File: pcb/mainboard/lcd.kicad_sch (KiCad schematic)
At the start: 15 parts

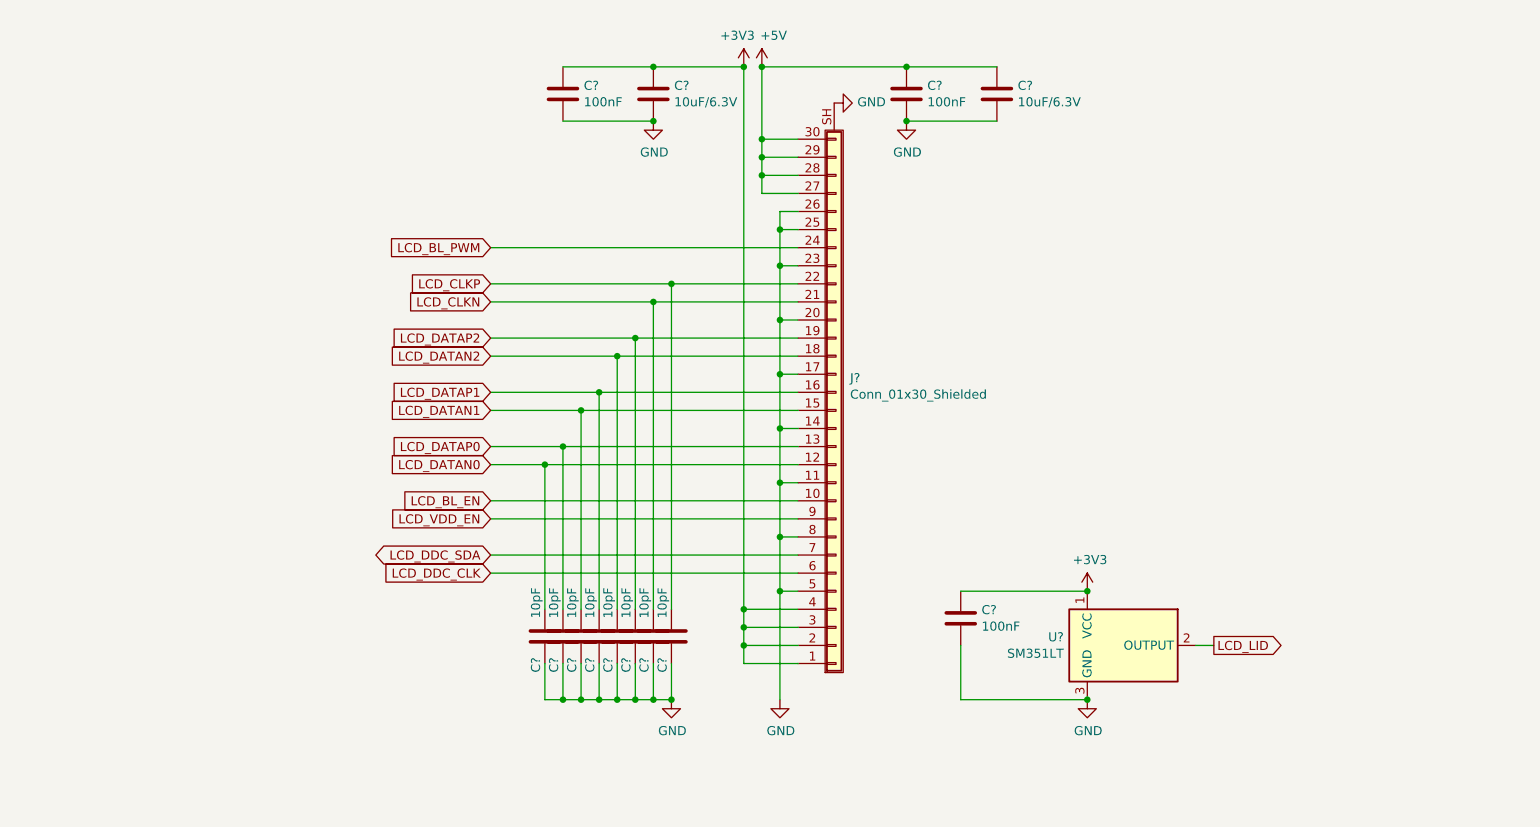
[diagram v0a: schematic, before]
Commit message: - Upgrade KiCad to latest version - Working on PM circuits - Initial USB Type-C support - Initial support for LCD
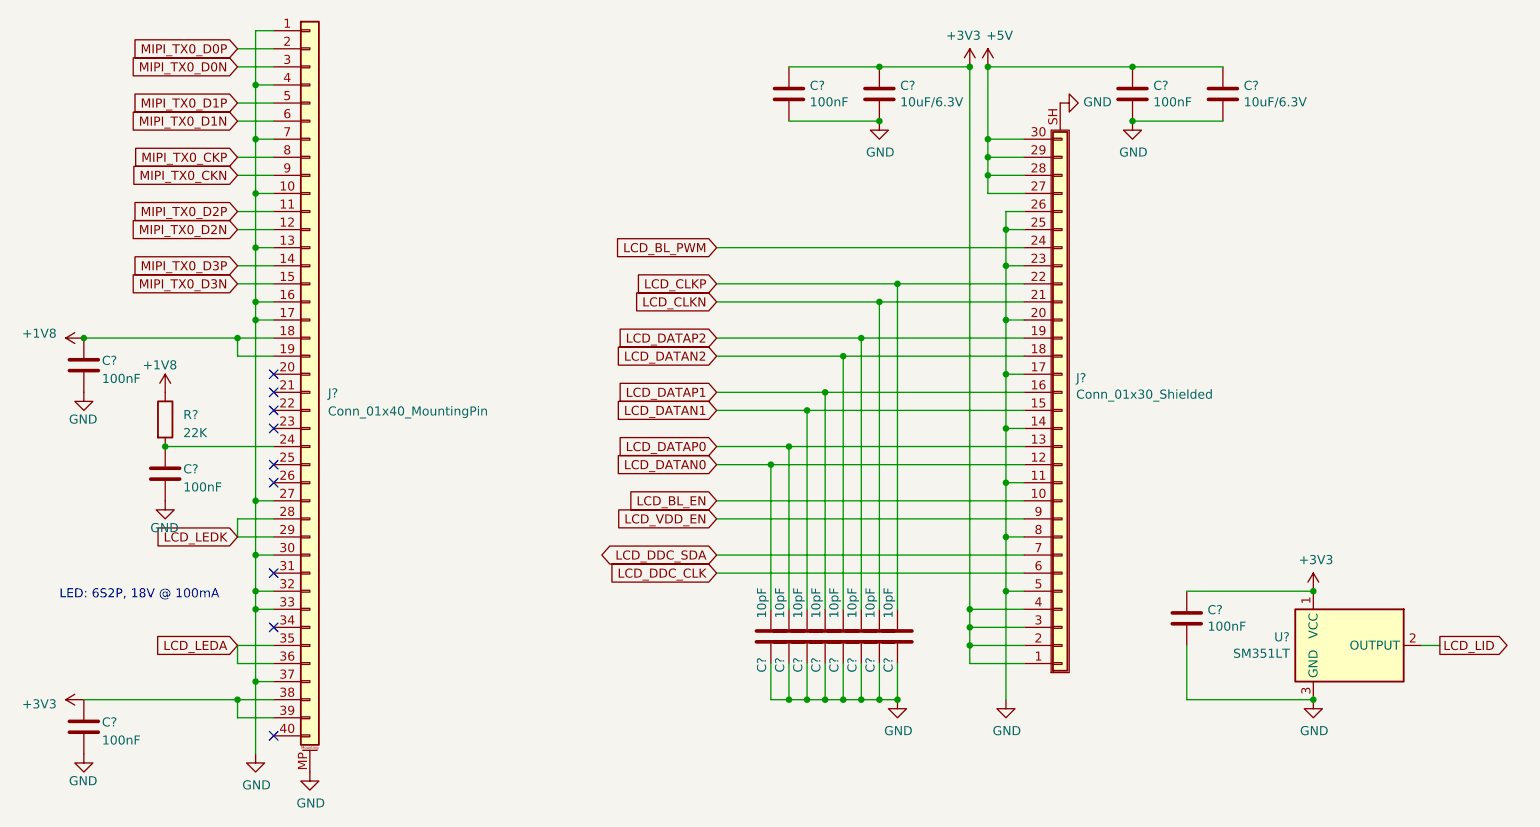
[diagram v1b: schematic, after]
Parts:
- added C? (x3): 100nF, symbol Device:C
- added J?: Conn_01x40_MountingPin, symbol Connector_Generic_MountingPin:Conn_01x40_MountingPin
- added R?: 22K, Resistor_SMD:R_0402_1005Metric, symbol Device:R
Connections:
- net +3V3: now also C?.1, J?.38 (Pin_38), J?.39 (Pin_39)
- net GND: now also C?.2, C?.2, C?.2, J?.1 (Pin_1), J?.10 (Pin_10), J?.13 (Pin_13), J?.16 (Pin_16), J?.17 (Pin_17), J?.27 (Pin_27), J?.30 (Pin_30), J?.32 (Pin_32), J?.33 (Pin_33), J?.37 (Pin_37), J?.4 (Pin_4), J?.7 (Pin_7), J?.MP (MountPin)
- new net: C?.1, J?.24 (Pin_24), R?.2
- new net +1V8: C?.1, J?.18 (Pin_18), J?.19 (Pin_19), R?.1
- new net LCD_LEDA: J?.35 (Pin_35), J?.36 (Pin_36)
- new net LCD_LEDK: J?.28 (Pin_28), J?.29 (Pin_29)
- new net MIPI_TX0_CKN: J?.9 (Pin_9)
- new net MIPI_TX0_CKP: J?.8 (Pin_8)
- new net MIPI_TX0_D0N: J?.3 (Pin_3)
- new net MIPI_TX0_D0P: J?.2 (Pin_2)
- new net MIPI_TX0_D1N: J?.6 (Pin_6)
- new net MIPI_TX0_D1P: J?.5 (Pin_5)
- new net MIPI_TX0_D2N: J?.12 (Pin_12)
- new net MIPI_TX0_D2P: J?.11 (Pin_11)
- new net MIPI_TX0_D3N: J?.15 (Pin_15)
- new net MIPI_TX0_D3P: J?.14 (Pin_14)
- no-connect marks 0 -> 9
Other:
- note added: "LED: 6S2P, 18V @ 100mA"
- moved on the sheet: C?, J?, U?

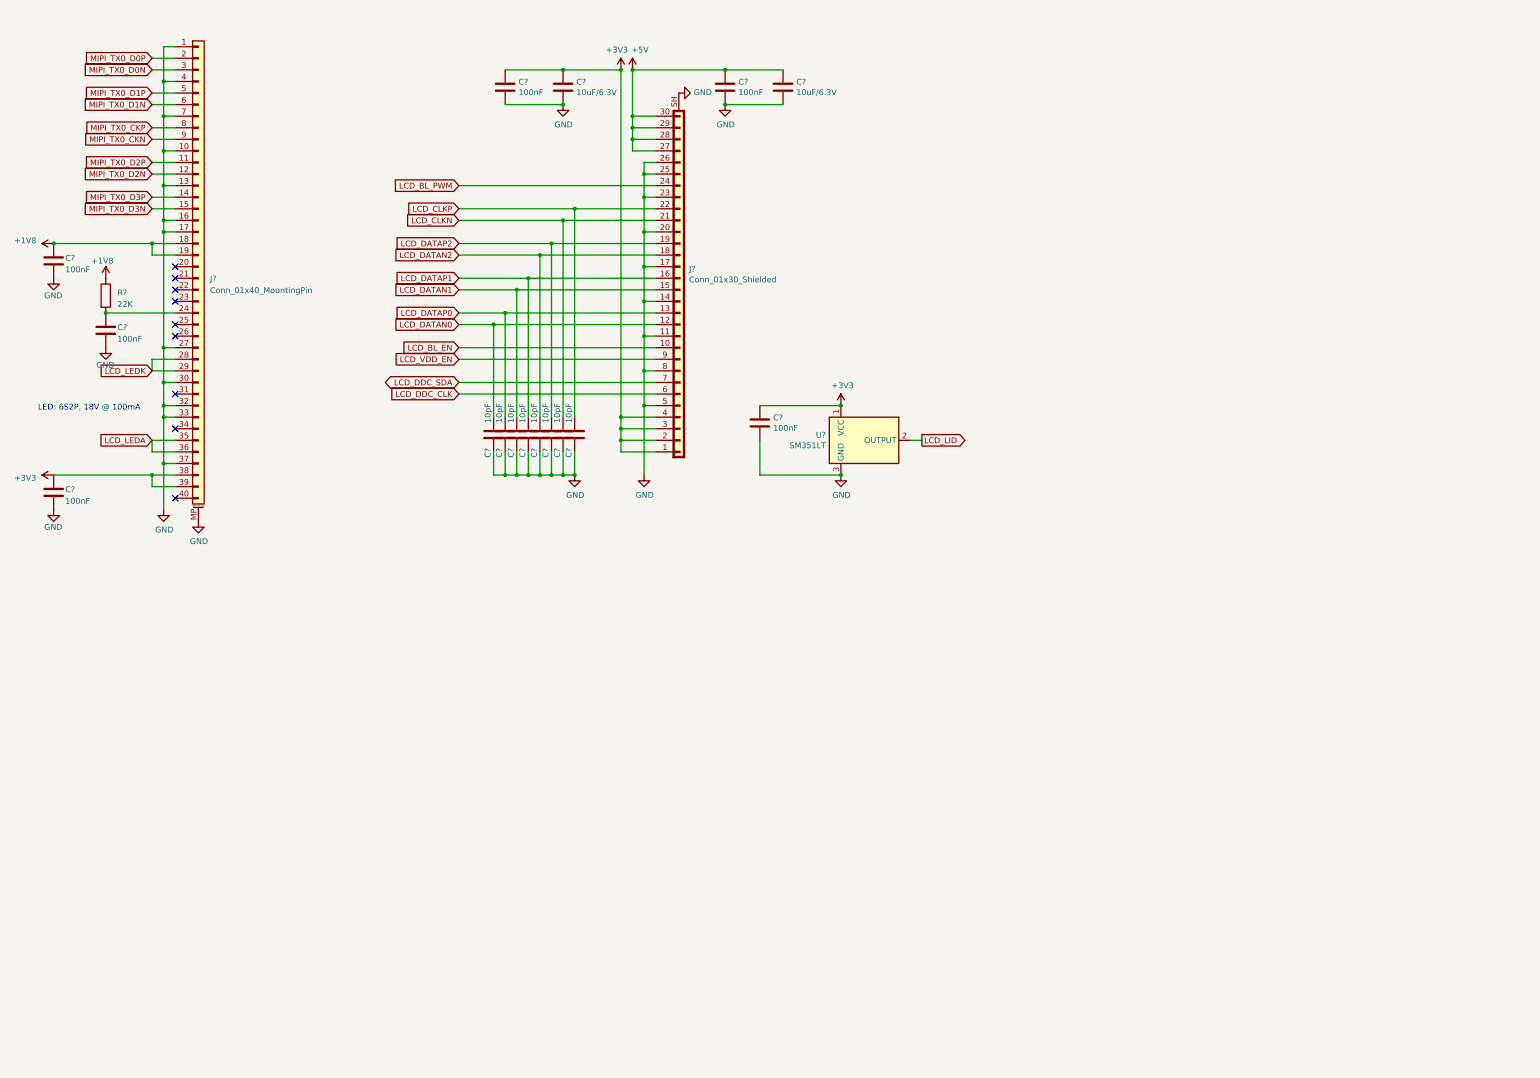
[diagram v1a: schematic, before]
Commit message: - pcb: working on r0p1 sch
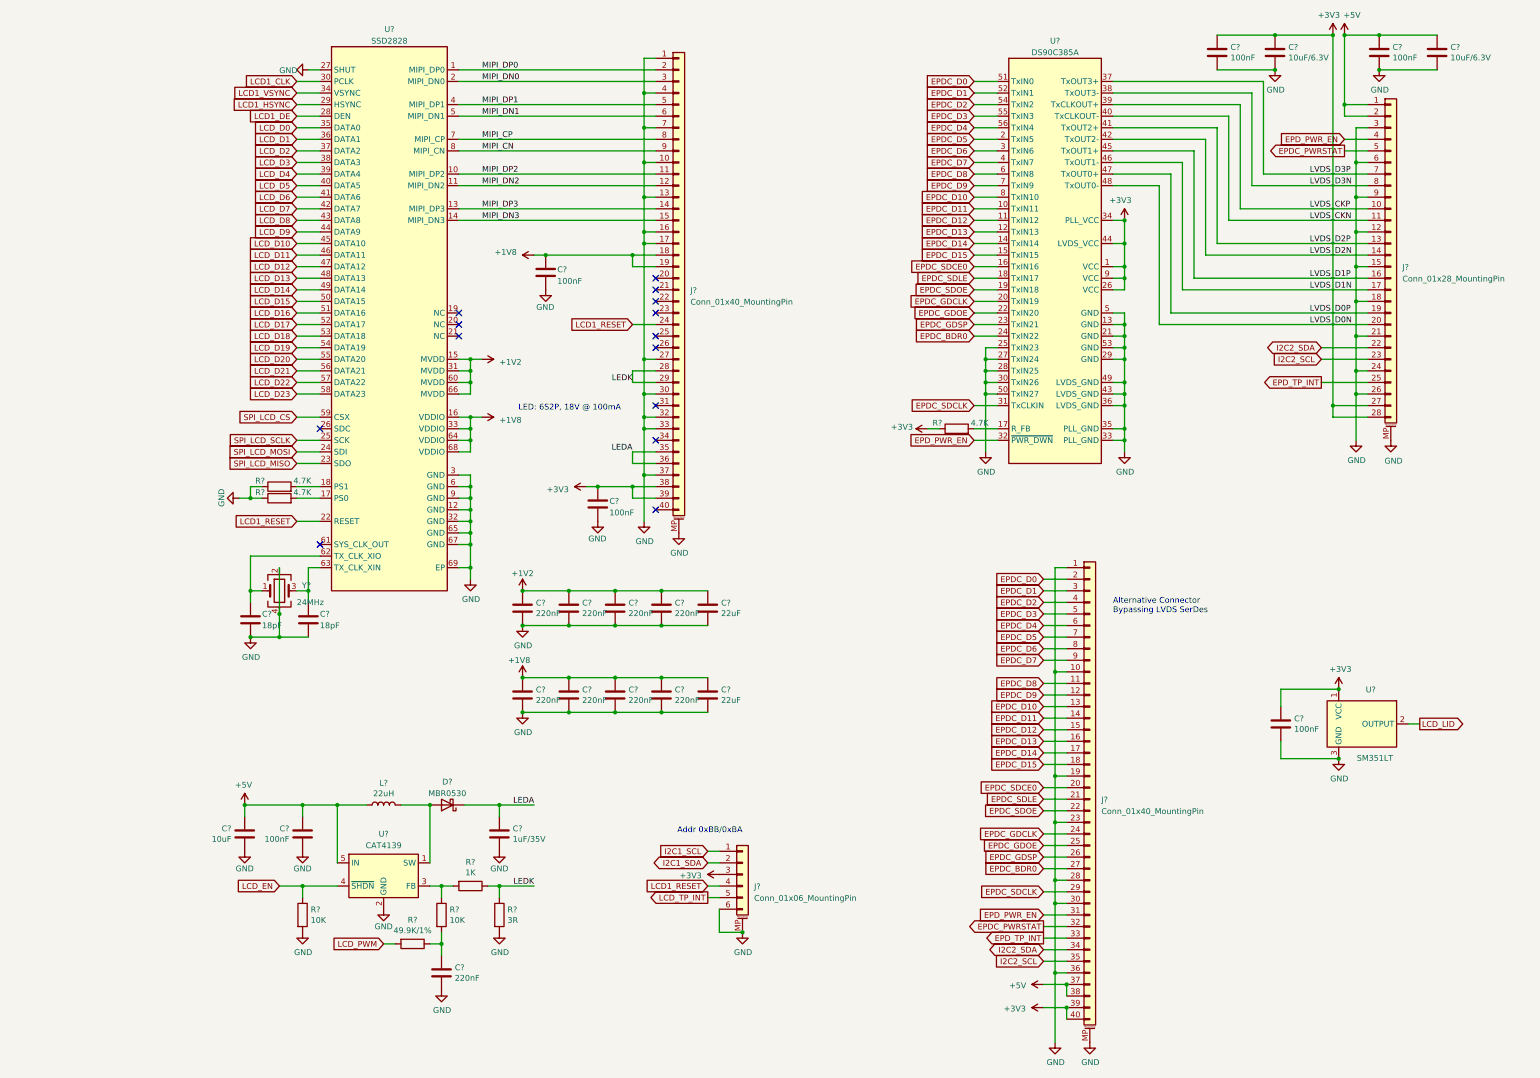
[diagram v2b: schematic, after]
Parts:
- removed C? (x8): 10pF, symbol Device:C
- removed C?: 100nF, symbol Device:C
- removed J?: Conn_01x30_Shielded, symbol Connector_Generic_Shielded:Conn_01x30_Shielded
- removed R?: 22K, Resistor_SMD:R_0402_1005Metric, symbol Device:R
- added C? (x9): 220nF, Capacitor_SMD:C_0402_1005Metric, symbol Device:C
- added C? (x2): 22uF, Capacitor_SMD:C_0603_1608Metric, symbol Device:C
- added C? (x2): 18pF, Capacitor_SMD:C_0603_1608Metric, symbol Device:C
- added C?: 1uF/35V, Capacitor_SMD:C_0603_1608Metric, symbol Device:C
- added C?: 100nF, Capacitor_SMD:C_0402_1005Metric, symbol Device:C
- added C?: 10uF, Capacitor_SMD:C_0603_1608Metric, symbol Device:C
- added D?: MBR0530, Diode_SMD:D_SOD-123, symbol Diode:MBR0530
- added J?: Conn_01x06_MountingPin, symbol Connector_Generic_MountingPin:Conn_01x06_MountingPin
- added J?: Conn_01x28_MountingPin, symbol Connector_Generic_MountingPin:Conn_01x28_MountingPin
- added J?: Conn_01x40_MountingPin, symbol Connector_Generic_MountingPin:Conn_01x40_MountingPin
- added L?: 22uH, Inductor_SMD:L_Vishay_IHLP-1212, symbol Device:L
- added R? (x3): 4.7K, Resistor_SMD:R_0402_1005Metric, symbol Device:R
- added R? (x2): 10K, Resistor_SMD:R_0402_1005Metric, symbol Device:R
- added R?: 3R, Resistor_SMD:R_0402_1005Metric, symbol Device:R
- added R?: 1K, Resistor_SMD:R_0402_1005Metric, symbol Device:R
- added R?: 49.9K/1%, Resistor_SMD:R_0402_1005Metric, symbol Device:R
- added U?: DS90C385A, Package_SO:TSSOP-56_6.1x14mm_P0.5mm, symbol symbols:DS90C385A
- added U?: CAT4139, Package_TO_SOT_SMD:SOT-23-5, symbol Regulator_Switching:AP3012
- added U?: SSD2828, Package_DFN_QFN:QFN-68-1EP_8x8mm_P0.4mm_EP5.2x5.2mm_ThermalVias, symbol symbols:SSD2828
- added Y?: 24MHz, Crystal:Crystal_SMD_3225-4Pin_3.2x2.5mm, symbol Device:Crystal_GND24
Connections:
- net +1V8: now also C?.1, C?.1, C?.1, C?.1, C?.1, U?.16 (VDDIO), U?.33 (VDDIO), U?.64 (VDDIO), U?.68 (VDDIO)
- net +3V3: now also J?.27 (Pin_27), J?.28 (Pin_28), J?.3 (Pin_3), J?.39 (Pin_39), J?.40 (Pin_40), R?.1, U?.1 (VCC), U?.26 (VCC), U?.34 (PLL_VCC), U?.44 (LVDS_VCC), U?.9 (VCC)
- net +5V: now also C?.2, C?.2, J?.1 (Pin_1), J?.2 (Pin_2), J?.37 (Pin_37), J?.38 (Pin_38), L?.1, U?.5 (IN)
- net GND: now also C?.1, C?.1, C?.1, C?.1, C?.1, C?.1, C?.2, C?.2, C?.2, C?.2, C?.2, C?.2, C?.2, C?.2, C?.2, C?.2, J?.1 (Pin_1), J?.10 (Pin_10), J?.12 (Pin_12), J?.15 (Pin_15), J?.18 (Pin_18), J?.19 (Pin_19), J?.21 (Pin_21), J?.23 (Pin_23), J?.24 (Pin_24), J?.26 (Pin_26), J?.28 (Pin_28), J?.3 (Pin_3), J?.30 (Pin_30), J?.36 (Pin_36), J?.6 (Pin_6), J?.6 (Pin_6), J?.9 (Pin_9), J?.MP (MountPin), J?.MP (MountPin), J?.MP (MountPin), R?.1, R?.1, R?.2, R?.2, U?.12 (GND), U?.13 (GND), U?.2 (GND), U?.21 (GND), U?.25 (TxIN23), U?.27 (SHUT), U?.27 (TxIN24), U?.28 (TxIN25), U?.29 (GND), U?.3 (GND), U?.30 (TxIN26), U?.32 (GND), U?.33 (PLL_GND), U?.35 (PLL_GND), U?.36 (LVDS_GND), U?.43 (LVDS_GND), U?.49 (LVDS_GND), U?.5 (GND), U?.50 (TxIN27), U?.53 (GND), U?.6 (GND), U?.65 (GND), U?.67 (GND), U?.69 (EP), U?.9 (GND), Y?.2, Y?.4
- net LCD1_RESET: now reaches J?.24 (Pin_24)
- net LCD1_RESET: now also J?.4 (Pin_4), U?.22 (RESET)
- net LCD_LEDA renamed LEDA
- net LEDA: now also C?.2, D?.1 (K)
- net LCD_LEDK renamed LEDK
- net LEDK: now also R?.1, R?.1
- net MIPI_TX0_CKN renamed MIPI_CN
- net MIPI_CN: now also U?.8 (MIPI_CN)
- net MIPI_TX0_CKP renamed MIPI_CP
- net MIPI_CP: now also U?.7 (MIPI_CP)
- net MIPI_TX0_D0N renamed MIPI_DN0
- net MIPI_DN0: now also U?.2 (MIPI_DN0)
- net MIPI_TX0_D0P renamed MIPI_DP0
- net MIPI_DP0: now also U?.1 (MIPI_DP0)
- net MIPI_TX0_D1N renamed MIPI_DN1
- net MIPI_DN1: now also U?.5 (MIPI_DN1)
- net MIPI_TX0_D1P renamed MIPI_DP1
- net MIPI_DP1: now also U?.4 (MIPI_DP1)
- net MIPI_TX0_D2N renamed MIPI_DN2
- net MIPI_DN2: now also U?.11 (MIPI_DN2)
- net MIPI_TX0_D2P renamed MIPI_DP2
- net MIPI_DP2: now also U?.10 (MIPI_DP2)
- net MIPI_TX0_D3N renamed MIPI_DN3
- net MIPI_DN3: now also U?.14 (MIPI_DN3)
- net MIPI_TX0_D3P renamed MIPI_DP3
- net MIPI_DP3: now also U?.13 (MIPI_DP3)
- new net: R?.2, U?.18 (PS1)
- new net: R?.2, U?.17 (R_FB)
- new net: D?.2 (A), L?.2, U?.1 (SW)
- new net: R?.1, R?.2, U?.3 (FB)
- new net: C?.2, R?.1, R?.2
- new net: C?.2, U?.63 (TX_CLK_XIN), Y?.3
- new net: C?.2, U?.62 (TX_CLK_XIO), Y?.1
- new net: R?.2, U?.17 (PS0)
- new net +1V2: C?.1, C?.1, C?.1, C?.1, C?.1, U?.15 (MVDD), U?.31 (MVDD), U?.60 (MVDD), U?.66 (MVDD)
- new net EPDC_BDR0: J?.27 (Pin_27), U?.24 (TxIN22)
- new net EPDC_D0: J?.2 (Pin_2), U?.51 (TxIN0)
- new net EPDC_D1: J?.3 (Pin_3), U?.52 (TxIN1)
- new net EPDC_D10: J?.13 (Pin_13), U?.8 (TxIN10)
- new net EPDC_D11: J?.14 (Pin_14), U?.10 (TxIN11)
- new net EPDC_D12: J?.15 (Pin_15), U?.11 (TxIN12)
- new net EPDC_D13: J?.16 (Pin_16), U?.12 (TxIN13)
- new net EPDC_D14: J?.17 (Pin_17), U?.14 (TxIN14)
- new net EPDC_D15: J?.18 (Pin_18), U?.15 (TxIN15)
- new net EPDC_D2: J?.4 (Pin_4), U?.54 (TxIN2)
- new net EPDC_D3: J?.5 (Pin_5), U?.55 (TxIN3)
- new net EPDC_D4: J?.6 (Pin_6), U?.56 (TxIN4)
- new net EPDC_D5: J?.7 (Pin_7), U?.2 (TxIN5)
- new net EPDC_D6: J?.8 (Pin_8), U?.3 (TxIN6)
- new net EPDC_D7: J?.9 (Pin_9), U?.4 (TxIN7)
- new net EPDC_D8: J?.11 (Pin_11), U?.6 (TxIN8)
- new net EPDC_D9: J?.12 (Pin_12), U?.7 (TxIN9)
- new net EPDC_GDCLK: J?.24 (Pin_24), U?.20 (TxIN19)
- new net EPDC_GDOE: J?.25 (Pin_25), U?.22 (TxIN20)
- new net EPDC_GDSP: J?.26 (Pin_26), U?.23 (TxIN21)
- new net EPDC_PWRSTAT: J?.32 (Pin_32), J?.5 (Pin_5)
- new net EPDC_SDCE0: J?.20 (Pin_20), U?.16 (TxIN16)
- new net EPDC_SDCLK: J?.29 (Pin_29), U?.31 (TxCLKIN)
- new net EPDC_SDLE: J?.21 (Pin_21), U?.18 (TxIN17)
- new net EPDC_SDOE: J?.22 (Pin_22), U?.19 (TxIN18)
- new net EPD_PWR_EN: J?.31 (Pin_31), J?.4 (Pin_4), U?.32 (~PWR_DWN)
- new net EPD_TP_INT: J?.25 (Pin_25), J?.33 (Pin_33)
- new net I2C1_SCL: J?.1 (Pin_1)
- new net I2C1_SDA: J?.2 (Pin_2)
- new net I2C2_SCL: J?.23 (Pin_23), J?.35 (Pin_35)
- new net I2C2_SDA: J?.22 (Pin_22), J?.34 (Pin_34)
- new net LCD1_CLK: U?.30 (PCLK)
- new net LCD1_DE: U?.28 (DEN)
- new net LCD1_HSYNC: U?.29 (HSYNC)
- new net LCD1_VSYNC: U?.34 (VSYNC)
- new net LCD_D0: U?.35 (DATA0)
- new net LCD_D1: U?.36 (DATA1)
- new net LCD_D10: U?.45 (DATA10)
- new net LCD_D11: U?.46 (DATA11)
- new net LCD_D12: U?.47 (DATA12)
- new net LCD_D13: U?.48 (DATA13)
- new net LCD_D14: U?.49 (DATA14)
- new net LCD_D15: U?.50 (DATA15)
- new net LCD_D16: U?.51 (DATA16)
- new net LCD_D17: U?.52 (DATA17)
- new net LCD_D18: U?.53 (DATA18)
- new net LCD_D19: U?.54 (DATA19)
- new net LCD_D2: U?.37 (DATA2)
- new net LCD_D20: U?.55 (DATA20)
- new net LCD_D21: U?.56 (DATA21)
- new net LCD_D22: U?.57 (DATA22)
- new net LCD_D23: U?.58 (DATA23)
- new net LCD_D3: U?.38 (DATA3)
- new net LCD_D4: U?.39 (DATA4)
- new net LCD_D5: U?.40 (DATA5)
- new net LCD_D6: U?.41 (DATA6)
- new net LCD_D7: U?.42 (DATA7)
- new net LCD_D8: U?.43 (DATA8)
- new net LCD_D9: U?.44 (DATA9)
- new net LCD_EN: R?.1, U?.4 (~SHDN~)
- new net LCD_PWM: R?.2
- new net LCD_TP_INT: J?.5 (Pin_5)
- new net LVDS_CKN: J?.11 (Pin_11), U?.40 (TxCLKOUT-)
- new net LVDS_CKP: J?.10 (Pin_10), U?.39 (TxCLKOUT+)
- new net LVDS_D0N: J?.20 (Pin_20), U?.48 (TxOUT0-)
- new net LVDS_D0P: J?.19 (Pin_19), U?.47 (TxOUT0+)
- new net LVDS_D1N: J?.17 (Pin_17), U?.46 (TxOUT1-)
- new net LVDS_D1P: J?.16 (Pin_16), U?.45 (TxOUT1+)
- new net LVDS_D2N: J?.14 (Pin_14), U?.42 (TxOUT2-)
- new net LVDS_D2P: J?.13 (Pin_13), U?.41 (TxOUT2+)
- new net LVDS_D3N: J?.8 (Pin_8), U?.38 (TxOUT3-)
- new net LVDS_D3P: J?.7 (Pin_7), U?.37 (TxOUT3+)
- new net SPI_LCD_CS: U?.59 (CSX)
- new net SPI_LCD_MISO: U?.23 (SDO)
- new net SPI_LCD_MOSI: U?.24 (SDI)
- new net SPI_LCD_SCLK: U?.25 (SCK)
- no-connect marks 9 -> 14
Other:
- note added: "Addr 0xBB/0xBA"
- note added: "Alternative Connector Bypassing LVDS SerDes"
- moved on the sheet: C?, J?, U?
